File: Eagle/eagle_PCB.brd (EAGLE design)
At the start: 65 x 61 mm, 14 parts, among them IC3 NE555, Q1 IRF740

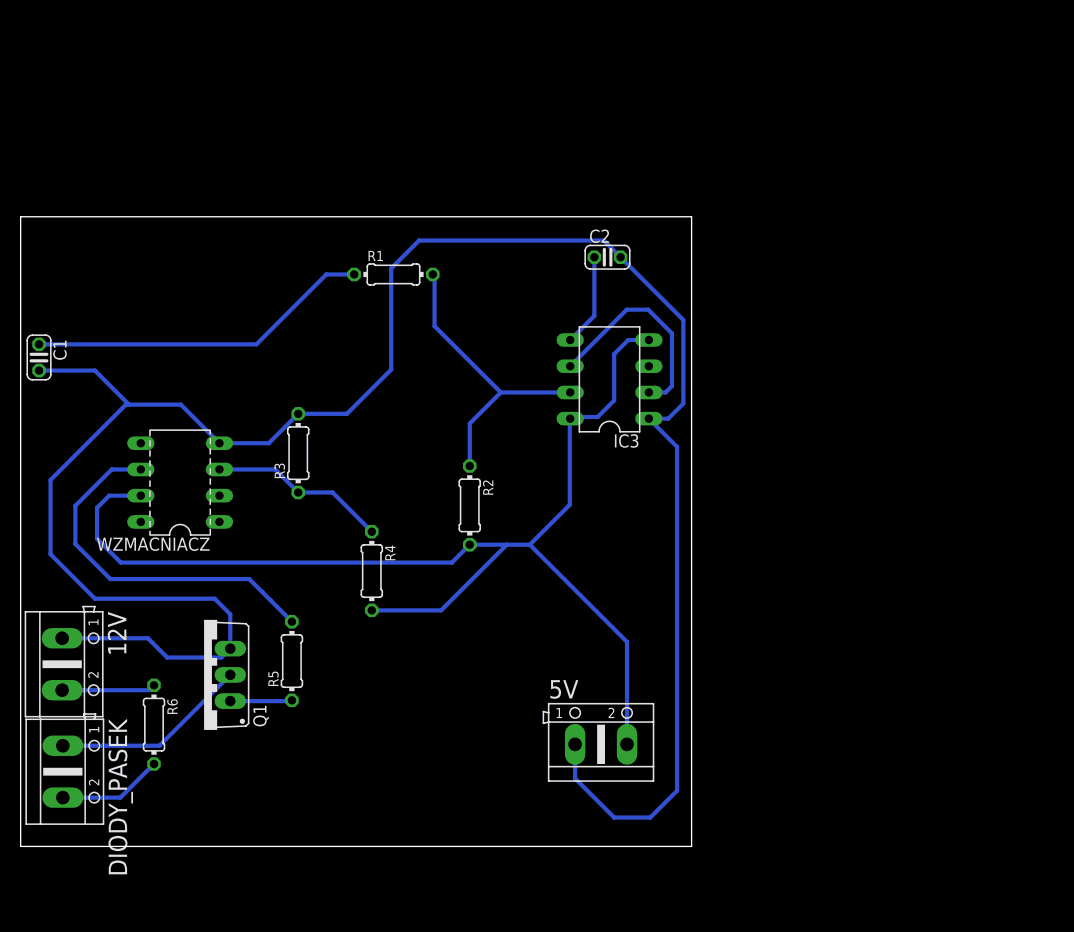
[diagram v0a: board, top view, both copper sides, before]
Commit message: update - eagle PCB ostatecza wersja
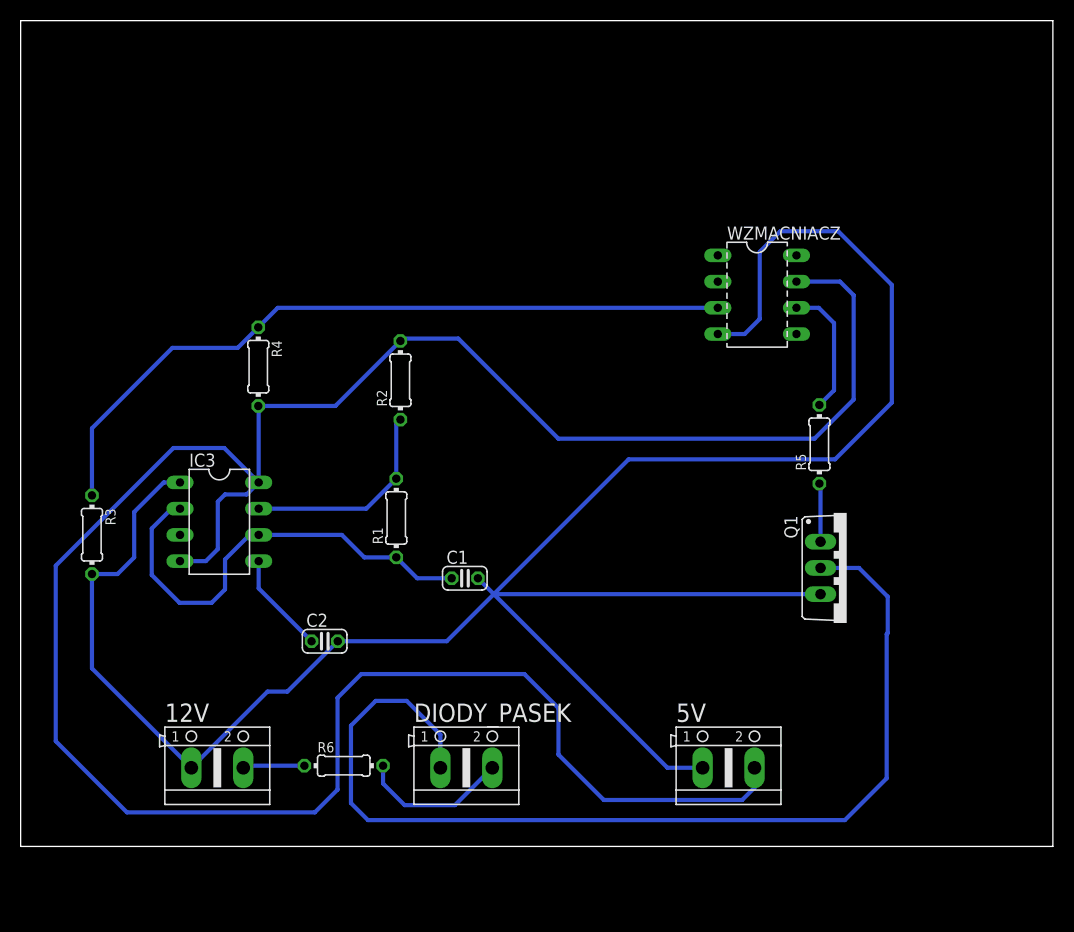
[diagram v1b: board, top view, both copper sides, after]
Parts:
- moved Q1 63.1 mm to (80.0, 27.0), turned to 270 degrees
- moved WZMACNIACZ 58.8 mm to (71.3, 53.5), turned to 270 degrees
- moved R5 55.2 mm to (77.4, 39.0)
- moved C1 46.5 mm to (43.0, 26.0), turned to 0 degrees
- moved C2 46.2 mm to (29.4, 19.9)
- moved IC3 40.2 mm to (19.2, 31.4), turned to 270 degrees
- moved DIODY_PASEK 39.1 mm to (43.2, 7.62), turned to 0 degrees
- moved R1 23.6 mm to (36.4, 31.8), turned to 90 degrees
- moved R4 22.7 mm to (23.0, 46.5)
- moved R3 21.5 mm to (6.91, 30.2), turned to 270 degrees
- moved R6 18.8 mm to (31.3, 7.82), turned to 0 degrees
- moved 12V 18.1 mm to (19.1, 7.62), turned to 0 degrees
- moved R2 13.9 mm to (36.8, 45.2), turned to 90 degrees
- moved 5V 12.6 mm to (68.6, 7.62)
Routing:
- net VCC: track 117.5 -> 237.3 mm
- net N$9: track 19.1 -> 101.3 mm
- net N$1: track 17.3 -> 72.0 mm
- net N$6: track 35.6 -> 12.8 mm
- net GND: track 205.8 -> 219.4 mm
- net N$5: track 54.0 -> 44.4 mm
- net N$2: track 29.3 -> 20.4 mm
- net N$8: track 10.2 -> 14.7 mm
- net +12V: track 9.10 -> 6.01 mm
- net N$4: track 8.99 -> 9.88 mm
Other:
- board size 65 x 61 mm -> 100 x 80 mm
